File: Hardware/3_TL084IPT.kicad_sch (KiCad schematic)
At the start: 23 parts, among them J9 Screw_Terminal_01x08, Q10 N_Mosfet, Q11 N_Mosfet, Q8 N_Mosfet, Q9 N_Mosfet, U13 TL084

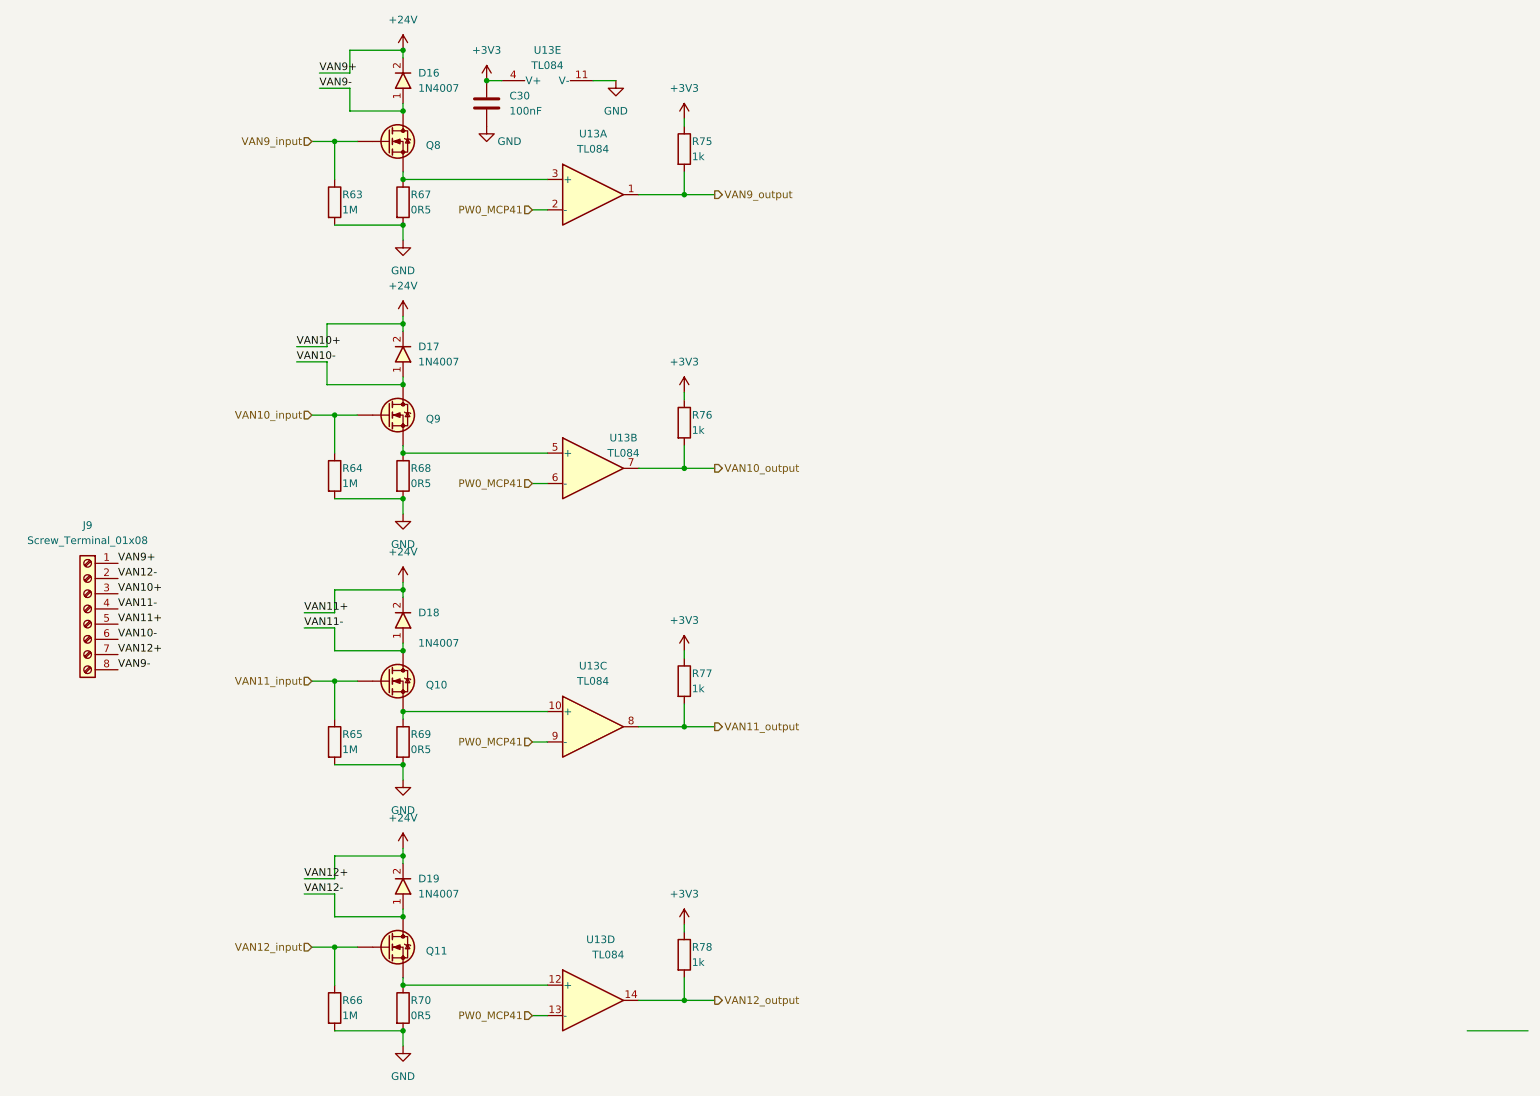
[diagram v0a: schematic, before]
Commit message: layout part 2
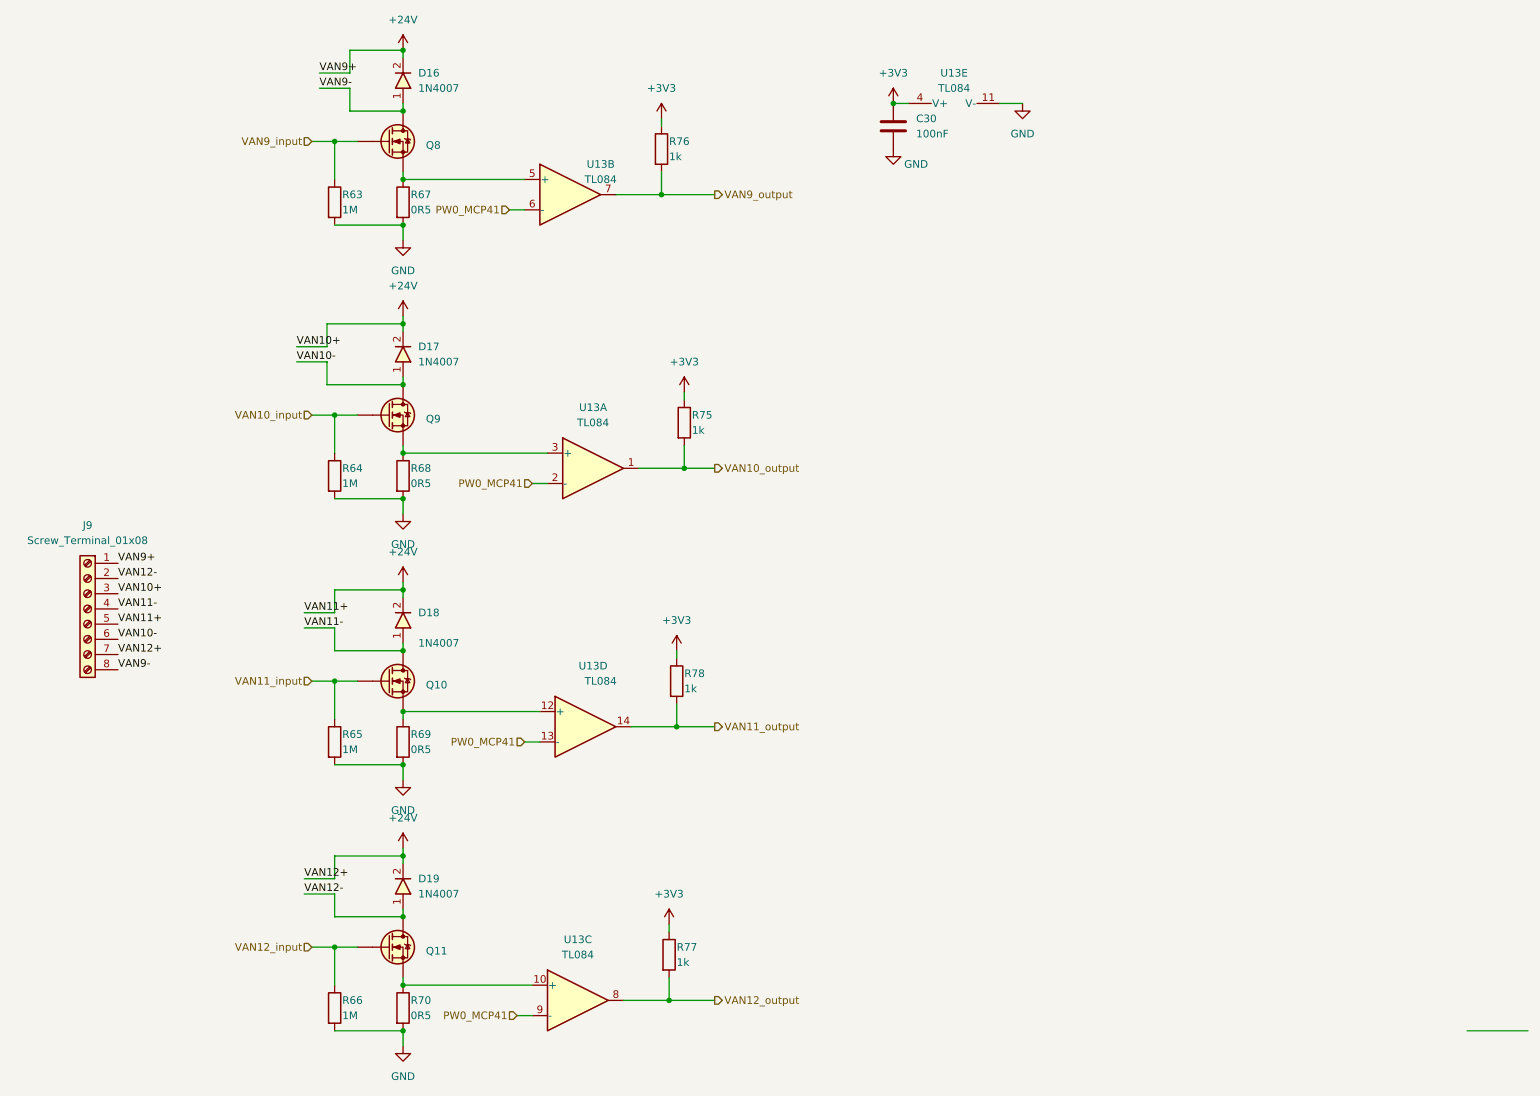
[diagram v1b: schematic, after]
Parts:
- D16, D17, D18, D19: footprint IVS_FOOTPRINTS:D_MiniMELF -> IVS_FOOTPRINTS:D_SOD323
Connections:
- net VAN10_output: now also R75.2, U13.1; no longer R76.2, U13.7
- net VAN11_output: now also R78.2, U13.14; no longer R77.2, U13.8
- net VAN12_output: now also R77.2, U13.8; no longer R78.2, U13.14
- net VAN9_output: now also R76.2, U13.7; no longer R75.2, U13.1
- net at Q10.2 (S), R69.1: now also U13.12 (+); no longer U13.10 (+)
- net at Q11.2 (S), R70.1: now also U13.10 (+); no longer U13.12 (+)
- net at Q9.2 (S), R68.1: now also U13.3 (+); no longer U13.5 (+)
- net at Q8.2 (S), R67.1: now also U13.5 (+); no longer U13.3 (+)
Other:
- moved on the sheet: C30, R75, R76, R77, R78, U13A, U13B, U13C, U13D, U13E
